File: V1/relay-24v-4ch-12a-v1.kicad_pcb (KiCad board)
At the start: 2 copper layers, 53 x 67.8 mm, 24 parts, among them J1 DB141V-2.54-2P, J2 DB141V-2.54-4P, J3 DB142V-5.08-4P, J4 DB142V-5.08-4P, K1 G5PZ-1A, K2 G5PZ-1A, K3 G5PZ-1A, K4 G5PZ-1A

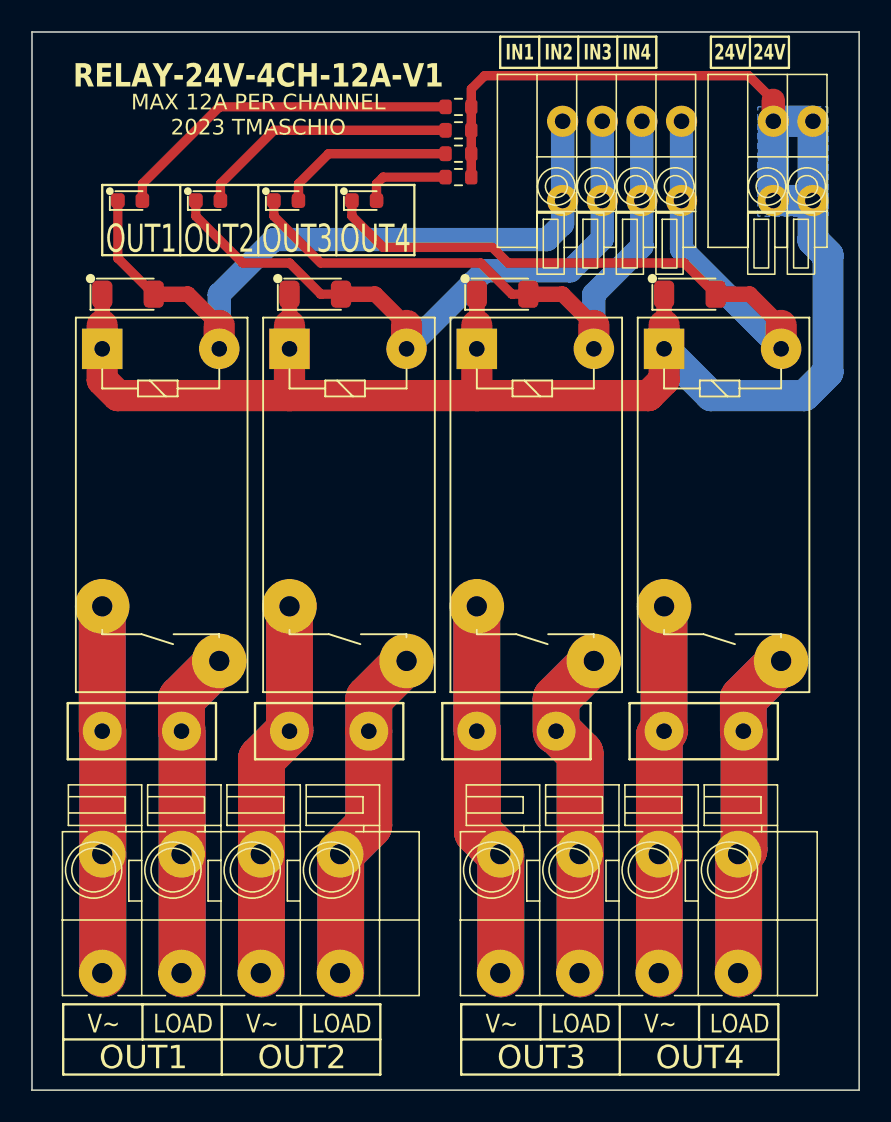
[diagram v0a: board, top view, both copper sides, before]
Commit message: Revision before manufacturing
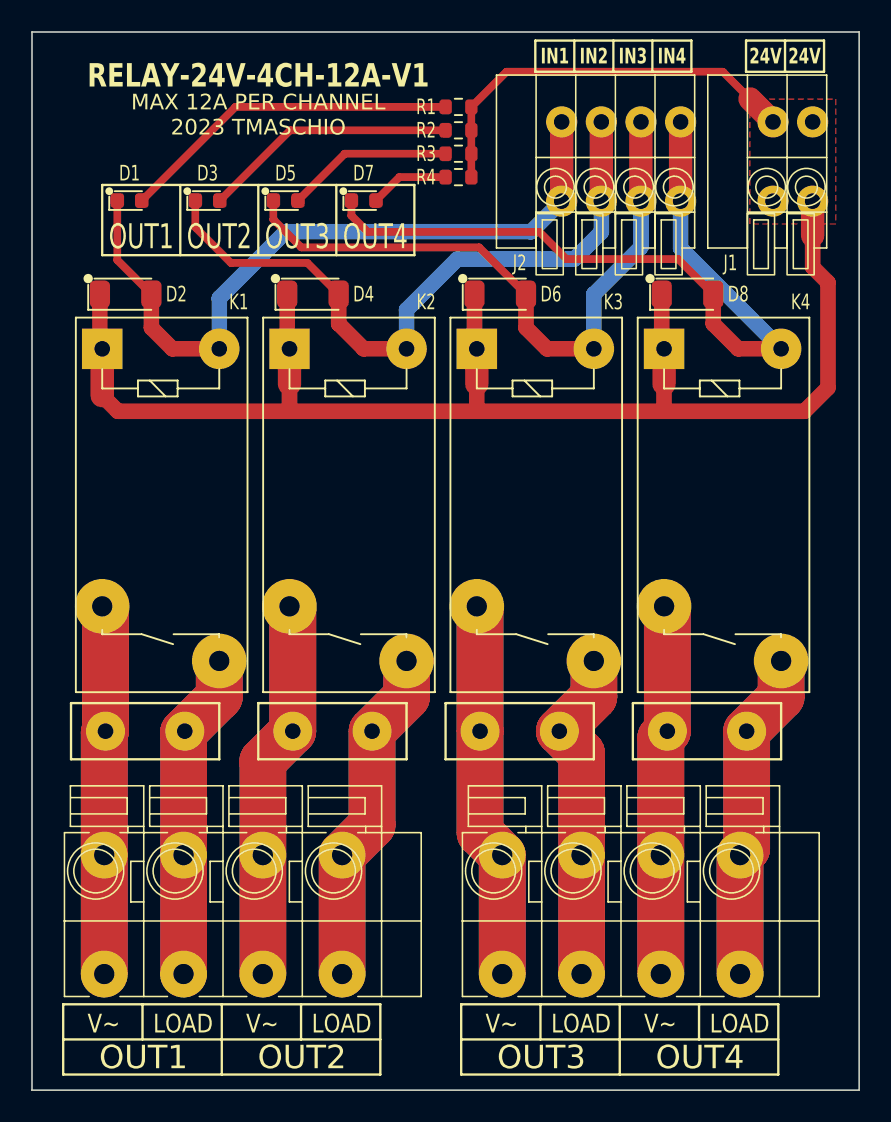
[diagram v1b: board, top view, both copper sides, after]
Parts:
- D1, D3, D5, D7: value GREEN -> WHITE
- R1, R2, R3, R4: value 6k8/100mW -> 10k/100mW
- moved K1 10.7 mm to (133.2, 92.5)
- moved K2 10.7 mm to (145.2, 92.5)
- moved K3 10.7 mm to (157.2, 92.5)
- moved K4 10.7 mm to (169.2, 92.5)
- moved J3 8.61 mm to (137.2, 118.8)
- moved J4 8.61 mm to (162.8, 118.8)
- moved J2 4.65 mm to (162.8, 70.5)
- moved J1 2.88 mm to (173.8, 70.5)
- moved RV1 2.75 mm to (132.2, 107.0)
- moved RV2 2.75 mm to (144.2, 107.0)
- moved RV3 2.75 mm to (156.2, 107.0)
- moved RV4 2.75 mm to (168.2, 107.0)
- moved D2 0.15 mm to (131.0, 79.0)
- moved D4 0.15 mm to (143.0, 79.0)
- moved D6 0.15 mm to (155.0, 79.0)
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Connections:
- net Net-(D1-A) renamed /LED1
- net Net-(D1-K) renamed /IN1
- net Net-(D3-A) renamed /LED2
- net Net-(D3-K) renamed /IN2
- net Net-(D5-A) renamed /LED3
- net Net-(D5-K) renamed /IN3
- net Net-(D7-A) renamed /LED4
- net Net-(D7-K) renamed /IN4
- net Net-(J3-Pin_1) renamed /OUT1PW
- net Net-(J3-Pin_2) renamed /OUT1LD
- net Net-(J3-Pin_3) renamed /OUT2PW
- net Net-(J3-Pin_4) renamed /OUT2LD
- net Net-(J4-Pin_1) renamed /OUT3PW
- net Net-(J4-Pin_2) renamed /OUT3LD
- net Net-(J4-Pin_3) renamed /OUT4PW
- net Net-(J4-Pin_4) renamed /OUT4LD
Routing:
- net +24V: track 127.2 -> 115.2 mm
- net /IN2: track 41.9 -> 43.7 mm
- net /IN1: track 47.4 -> 46.8 mm
- net /LED3: track 11.3 -> 10.7 mm
- net /LED4: track 5.68 -> 5.08 mm
- net /LED2: track 16.9 -> 16.3 mm
- net /LED1: track 22.5 -> 21.9 mm
- added copper zone on F.Cu, net +24V
- removed copper zone on B.Cu, net +24V
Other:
- rule pad_to_mask_clearance: 0 -> 0.1
